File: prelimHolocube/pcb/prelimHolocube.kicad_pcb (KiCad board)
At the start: 2 copper layers, 28.2 x 51.4 mm, 43 parts

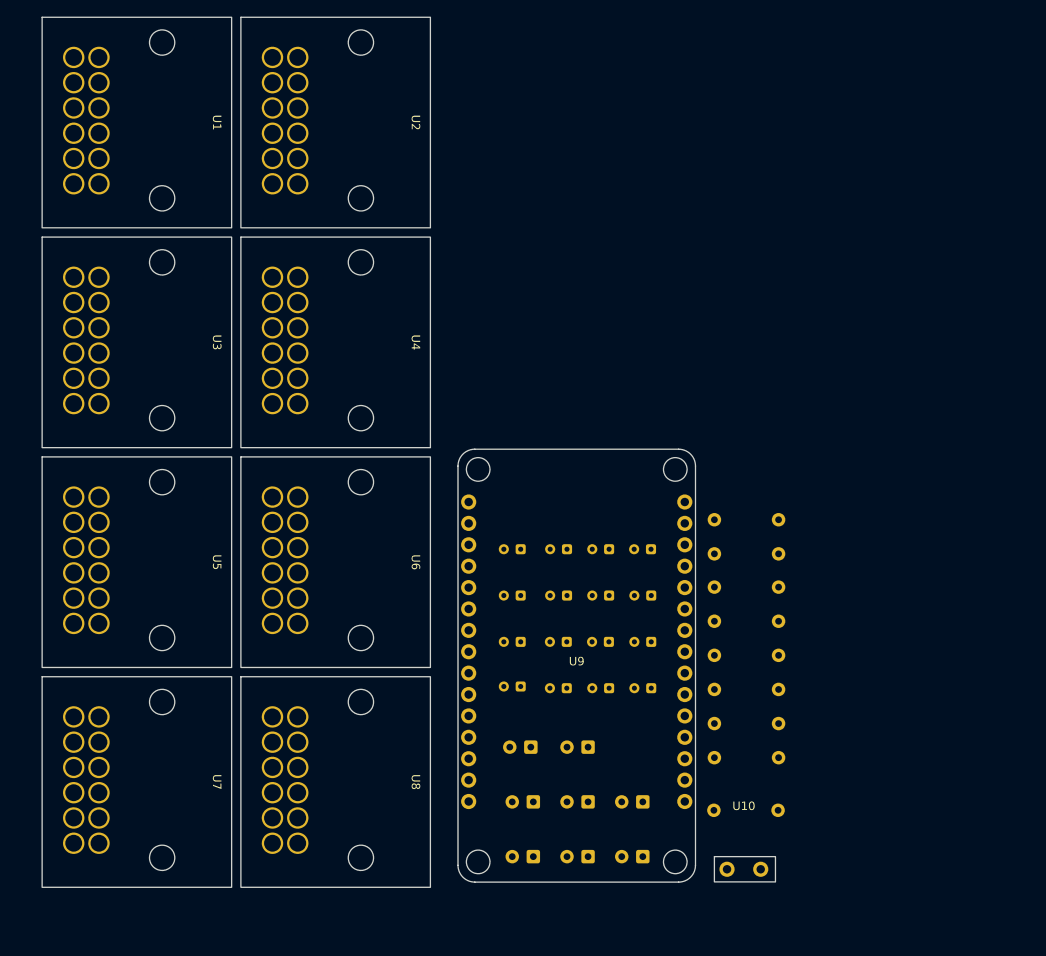
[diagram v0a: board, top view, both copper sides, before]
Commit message: finish pcb
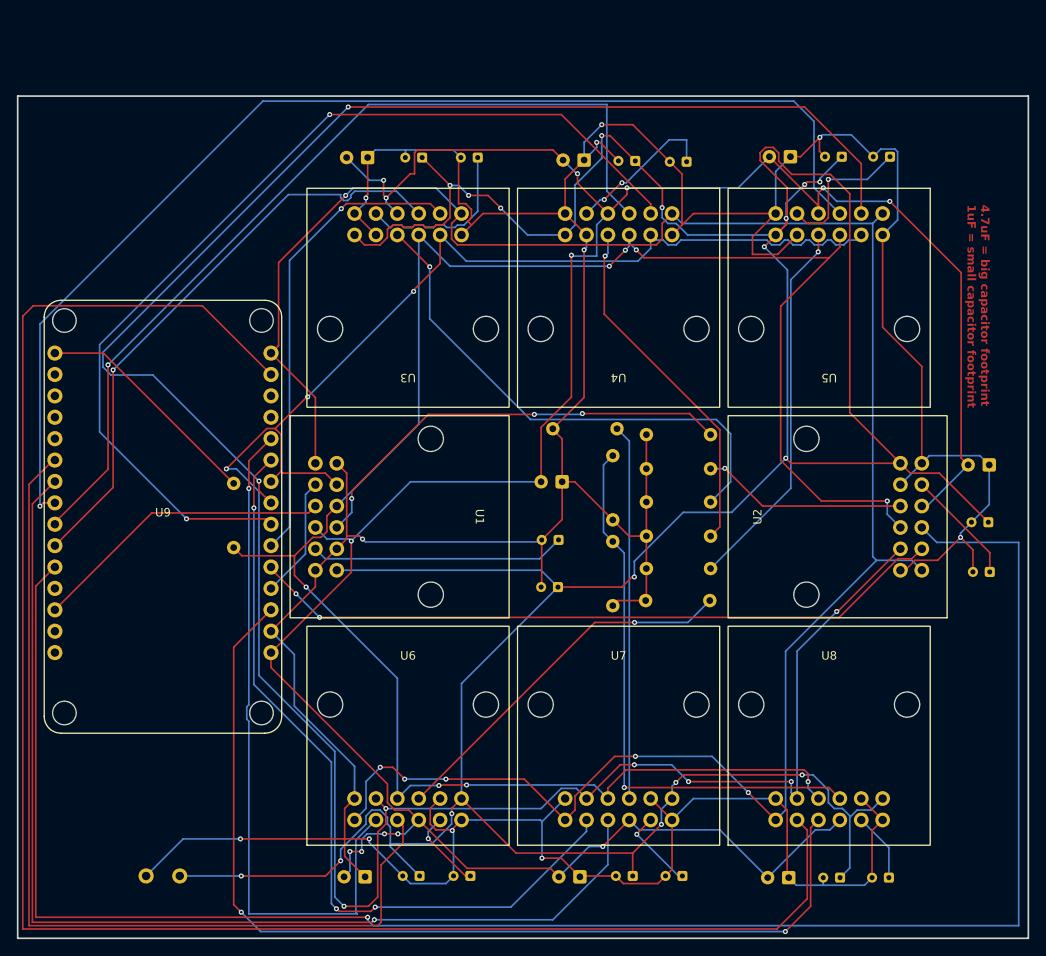
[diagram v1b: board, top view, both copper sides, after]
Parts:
- removed C25, C27: 1uF, Capacitor_THT:CP_Radial_D5.0mm_P2.50mm
- removed C26, C28, C29, C30: 4.7uF, Capacitor_THT:CP_Radial_D4.0mm_P2.00mm
- removed the U4 at (127.2, 81.5)
- added C16: 4.7uF, Capacitor_THT:CP_Radial_D4.0mm_P2.00mm, B.Cu at (137.2, 144.9)
- added C17: 4.7uF, Capacitor_THT:CP_Radial_D4.0mm_P2.00mm, B.Cu at (193.0, 59.5)
- added C18: 4.7uF, Capacitor_THT:CP_Radial_D4.0mm_P2.00mm, B.Cu at (143.2, 144.9)
- added C7: 1uF, Capacitor_THT:CP_Radial_D5.0mm_P2.50mm, B.Cu at (131.0, 59.6)
- added C8: 4.7uF, Capacitor_THT:CP_Radial_D4.0mm_P2.00mm, B.Cu at (137.5, 59.6)
- added C9: 4.7uF, Capacitor_THT:CP_Radial_D4.0mm_P2.00mm, B.Cu at (144.1, 59.6)
- added R6: 1M, Resistor_THT:R_Axial_DIN0207_L6.3mm_D2.5mm_P7.62mm_Horizontal, B.Cu at (171.7, 108.4)
- added U3: ~, transparent_oled_display:surenoo-1.12in-128x128, F.Cu at (135.8, 76.2)
- C15: value 4.7uF -> 1uF; footprint Capacitor_THT:CP_Radial_D4.0mm_P2.00mm -> Capacitor_THT:CP_Radial_D5.0mm_P2.50mm
- U10: moved to B.Cu
- moved U5 88.0 mm to (185.8, 76.2), turned to -90 degrees
- moved C10 82.7 mm to (156.7, 59.9)
- moved C13 80.3 mm to (181.2, 59.5)
- moved U2 75.8 mm to (186.8, 102.2), turned to 180 degrees
- moved R3 75.4 mm to (115.1, 98.3), turned to -90 degrees
- moved U10 69.0 mm to (106.7, 144.9), turned to 180 degrees
- moved C11 62.7 mm to (162.8, 60.0)
- moved C14 59.0 mm to (187.3, 59.5)
- moved U8 58.9 mm to (185.8, 128.2), turned to 90 degrees
- moved C4 58.2 mm to (204.8, 96.1)
- moved U7 57.5 mm to (160.8, 128.2), turned to 90 degrees
- moved U4 57.4 mm to (160.8, 76.2), turned to -90 degrees
- moved U1 56.2 mm to (134.8, 102.2)
- moved U9 52.2 mm to (106.7, 102.2)
- moved C12 51.7 mm to (168.9, 60.1)
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- renumbered U3 to U4
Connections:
- C15 pad 1: Net-(U4-VCOMH) (its old number) -> GND
- C15 pad 2: GND -> +3.3V
- C23 pad 1: Net-(U5-VCOMH) -> Net-(U7-VCOMH)
- C24 pad 1: Net-(U7-VCOMH) -> Net-(U8-VCOMH)
- R7 pad 1: Net-(U5-IREF) -> Net-(U6-IREF)
- R9 pad 1: Net-(U6-IREF) -> Net-(U8-IREF)
- U4 pad 4: A03 -> A04
- U4 pad 6: CS3 -> CS4
- U4 pad 7: Net-(U3-IREF) -> Net-(U4-IREF)
- U6 pad 4: A06 -> A07
- U6 pad 6: CS6 -> CS7
- U7 pad 4: A07 -> A06
- U7 pad 6: CS7 -> CS6
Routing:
- net GND: track 0.00 -> 522.7 mm, vias 0 -> 11
- net +12V: track 0.00 -> 423.0 mm, vias 0 -> 17
- net +3.3V: track 0.00 -> 318.1 mm, vias 0 -> 13
- net SCL: track 0.00 -> 274.3 mm, vias 0 -> 9
- net SI: track 0.00 -> 257.7 mm, vias 0 -> 6
- net RES: track 0.00 -> 244.7 mm, vias 0 -> 8
- net CS2: track 0.00 -> 217.6 mm, vias 0 -> 1
- net A08: track 0.00 -> 210.6 mm
- net A05: track 0.00 -> 139.9 mm, vias 0 -> 2
- net CS5: track 0.00 -> 139.6 mm, vias 0 -> 1
- net CS6: track 0.00 -> 129.9 mm, vias 0 -> 1
- net CS8: track 0.00 -> 118.5 mm, vias 0 -> 2
- net A04: track 0.00 -> 117.5 mm, vias 0 -> 2
- net CS7: track 0.00 -> 112.3 mm
- net CS4: track 0.00 -> 107.6 mm, vias 0 -> 1
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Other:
- board size 28.2 x 51.4 mm -> 120 x 100 mm
- board text added: "4.7uF = big capacitor footprint 1uF = small capacitor footprint"
- board text removed: "1M ^ 10k v"
- board text removed: "4.7uF ^ 1uF v"
